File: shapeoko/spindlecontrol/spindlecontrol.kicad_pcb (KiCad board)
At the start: 2 copper layers, 61 x 50.8 mm, 10 parts, among them J1 Control, J2 Mains, J3 Relay coil, Q1 BC547, U1 PC817

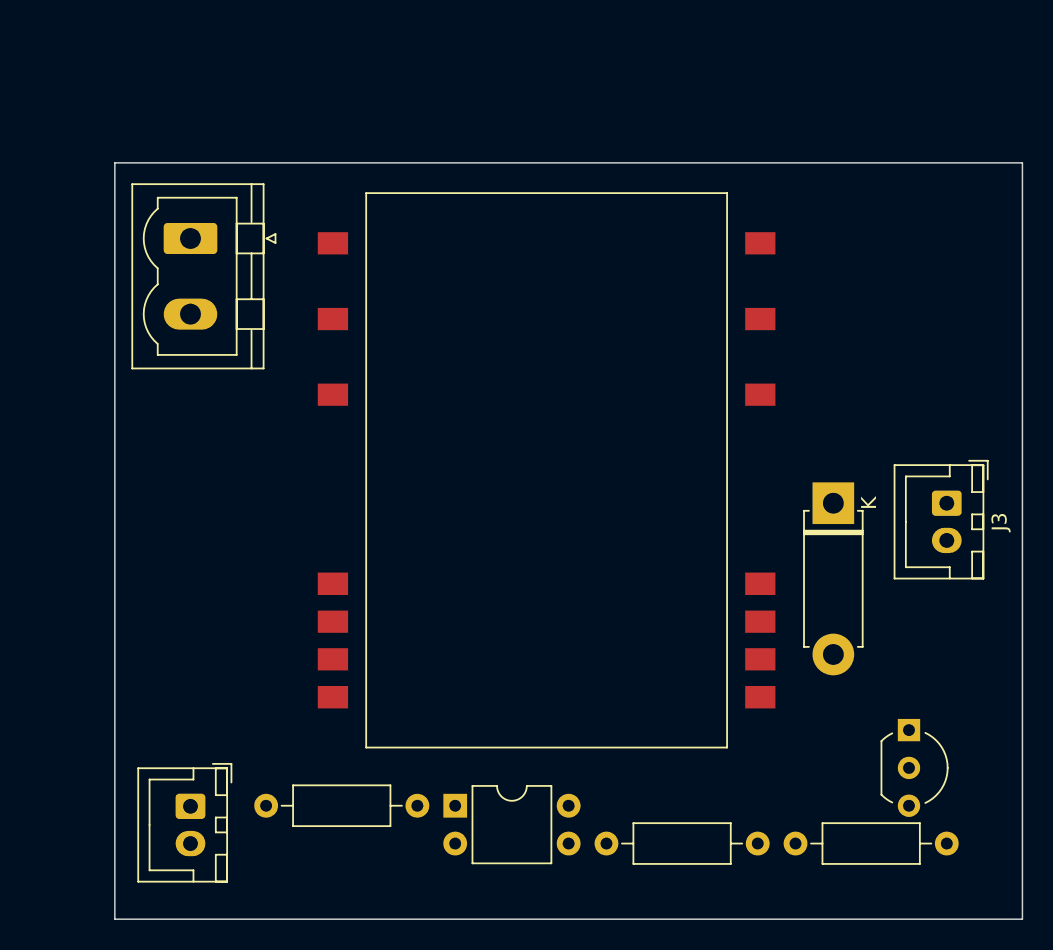
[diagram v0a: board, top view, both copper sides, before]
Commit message: Route.
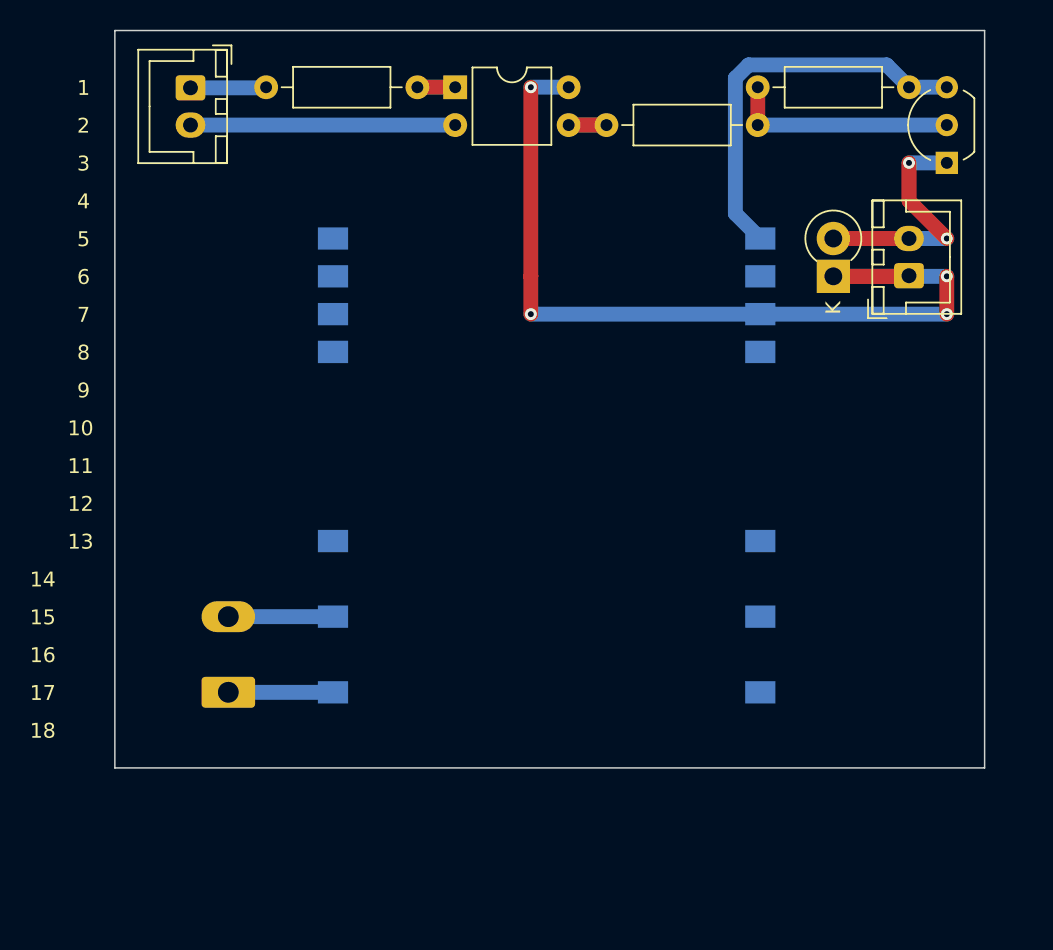
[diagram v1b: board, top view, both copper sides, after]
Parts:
- D1: footprint Diode_THT:D_5W_P10.16mm_Horizontal -> Diode_THT:D_DO-15_P2.54mm_Vertical_KathodeUp
- J2: footprint Connector_Phoenix_MSTB:PhoenixContact_MSTBVA_2,5_2-G-5,08_1x02_P5.08mm_Vertical -> Connector_Phoenix_MSTB:PhoenixContact_MSTBA_2,5_2-G-5,08_1x02_P5.08mm_Horizontal; moved to B.Cu
- PS1: moved to B.Cu
- moved R3 50.9 mm to (76.2, 40.6)
- moved R1 48.3 mm to (43.2, 40.6)
- moved U1 48.3 mm to (55.9, 40.6)
- moved J1 48.3 mm to (38.1, 40.7)
- moved R2 48.3 mm to (66.0, 43.2)
- moved Q1 38.2 mm to (88.9, 45.7), turned to 90 degrees
- moved J2 30.6 mm to (40.6, 81.3), turned to 90 degrees
- moved J3 15.5 mm to (86.4, 53.3), turned to 90 degrees
- moved D1 15.2 mm to (81.3, 53.3), turned to 90 degrees
- moved PS1 0.33 mm to (62.0, 66.0)
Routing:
- net +24V: track 0.00 -> 61.0 mm, vias 0 -> 4
- net GND: track 0.00 -> 26.7 mm
- net Net-(D1-A): track 0.00 -> 21.4 mm, vias 0 -> 2
- net Net-(J1-Pin_2): track 0.00 -> 17.8 mm
- net Net-(Q1-B): track 0.00 -> 15.2 mm
- net N: track 0.00 -> 7.03 mm
- net L: track 0.00 -> 7.03 mm
- net Net-(J1-Pin_1): track 0.00 -> 5.15 mm
- net Net-(R2-Pad1): track 0.00 -> 5.08 mm
- net Net-(R1-Pad2): track 0.00 -> 5.08 mm
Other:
- board size 61 x 50.8 mm -> 58.4 x 49.5 mm
- board text added: "1"
- board text added: "10"
- board text added: "11"
- board text added: "12"
- board text added: "13"
- board text added: "14"
- board text added: "15"
- board text added: "16"
- board text added: "17"
- board text added: "18"
- board text added: "2"
- board text added: "20"
- board text added: "22"
- board text added: "24"
- board text added: "3"
- board text added: "4"
- board text added: "5"
- board text added: "6"
- board text added: "7"
- board text added: "8"
- board text added: "9"

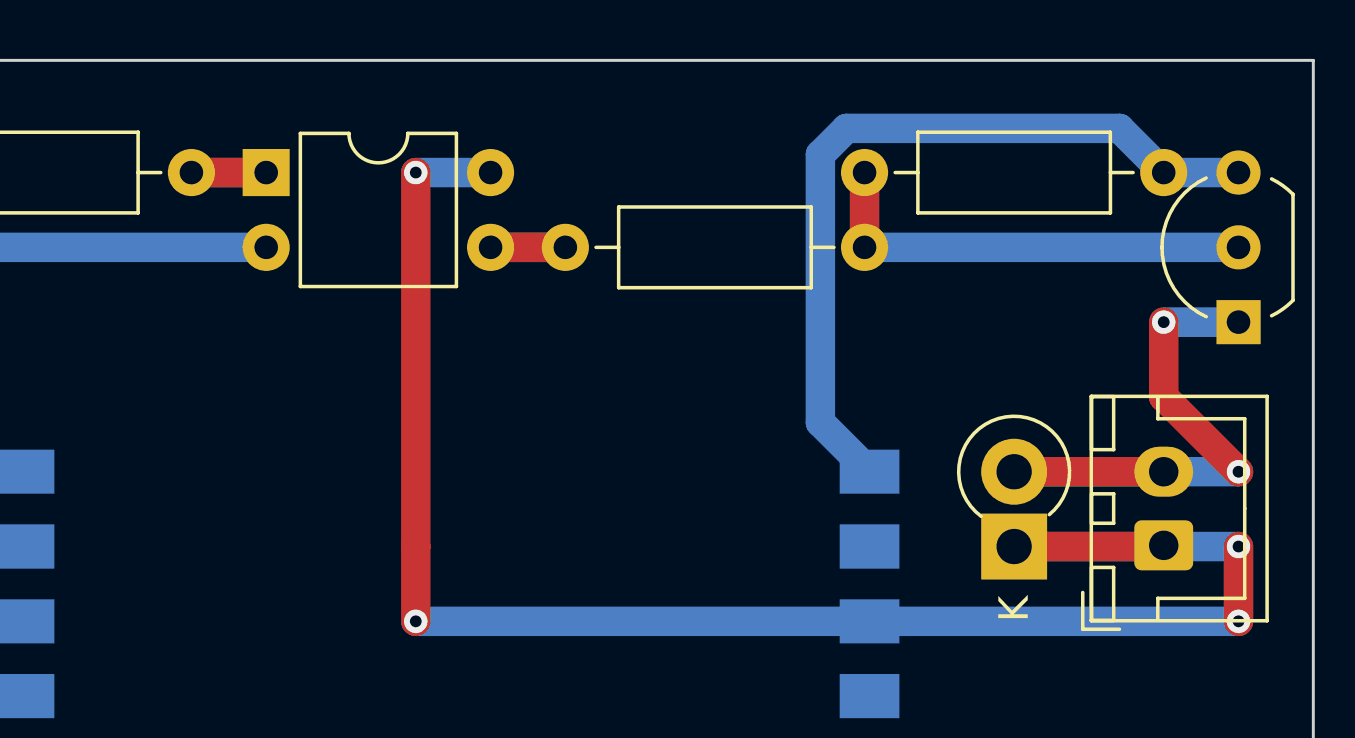
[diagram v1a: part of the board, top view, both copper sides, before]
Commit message: Add
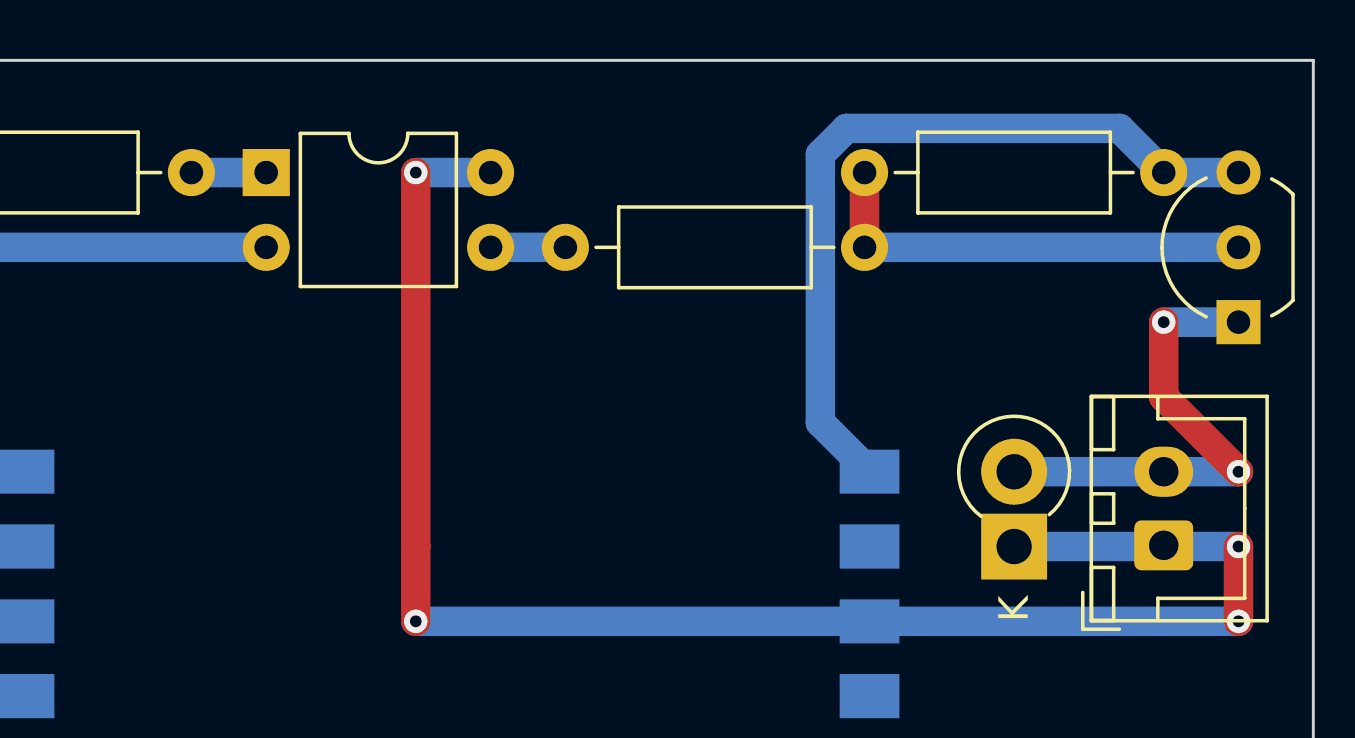
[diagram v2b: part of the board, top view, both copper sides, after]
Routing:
- net Net-(D1-A): track 21.4 -> 16.3 mm
- net +24V: track 61.0 -> 56.0 mm
- net Net-(R2-Pad1): track 5.08 -> 2.54 mm
- net Net-(R1-Pad2): track 5.08 -> 2.54 mm
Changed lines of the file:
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@@
   (segment (start 60.96 55.88) (end 60.96 53.34) (width 1) (layer "F.Cu") (net 1))
   (segment (start 88.9 55.88) (end 88.9 53.34) (width 1) (layer "F.Cu") (net 1))
-  (segment (start 81.28 53.34) (end 86.32 53.34) (width 1) (layer "F.Cu") (net 1))
   (segment (start 60.96 53.34) (end 60.96 40.64) (width 1) (layer "F.Cu") (net 1))
   (via (at 60.96 55.88) (size 0.8) (drill 0.4) (layers "F.Cu" "B.Cu") (net 1))
@@
   (segment (start 86.36 48.26) (end 88.9 50.8) (width 1) (layer "F.Cu") (net 2))
   (segment (start 86.36 45.72) (end 86.36 48.26) (width 1) (layer "F.Cu") (net 2))
-  (segment (start 81.28 50.8) (end 86.36 50.8) (width 1) (layer "F.Cu") (net 2))
   (via (at 86.36 45.72) (size 0.8) (drill 0.4) (layers "F.Cu" "B.Cu") (net 2))
   (via (at 88.9 50.8) (size 0.8) (drill 0.4) (layers "F.Cu" "B.Cu") (net 2))
@@
   (segment (start 76.2 40.64) (end 76.2 43.18) (width 1) (layer "F.Cu") (net 8))
   (segment (start 76.2 43.18) (end 88.9 43.18) (width 1) (layer "B.Cu") (net 8))
-  (segment (start 55.88 40.64) (end 53.34 40.64) (width 1) (layer "F.Cu") (net 9))
   (segment (start 53.34 40.64) (end 55.88 40.64) (width 1) (layer "B.Cu") (net 9))
-  (segment (start 63.5 43.18) (end 66.04 43.18) (width 1) (layer "F.Cu") (net 10))
   (segment (start 63.5 43.18) (end 66.04 43.18) (width 1) (layer "B.Cu") (net 10))
   (group "" (id 559b0eab-46f0-4a7e-ac66-a8071223d0b4)
